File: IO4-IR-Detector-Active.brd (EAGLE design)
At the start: 50 x 50 mm, 32 parts, among them Q1 NPN-2222, Q2 NPN-2222, Q3 NPN-2222, Q4 NPN-2222

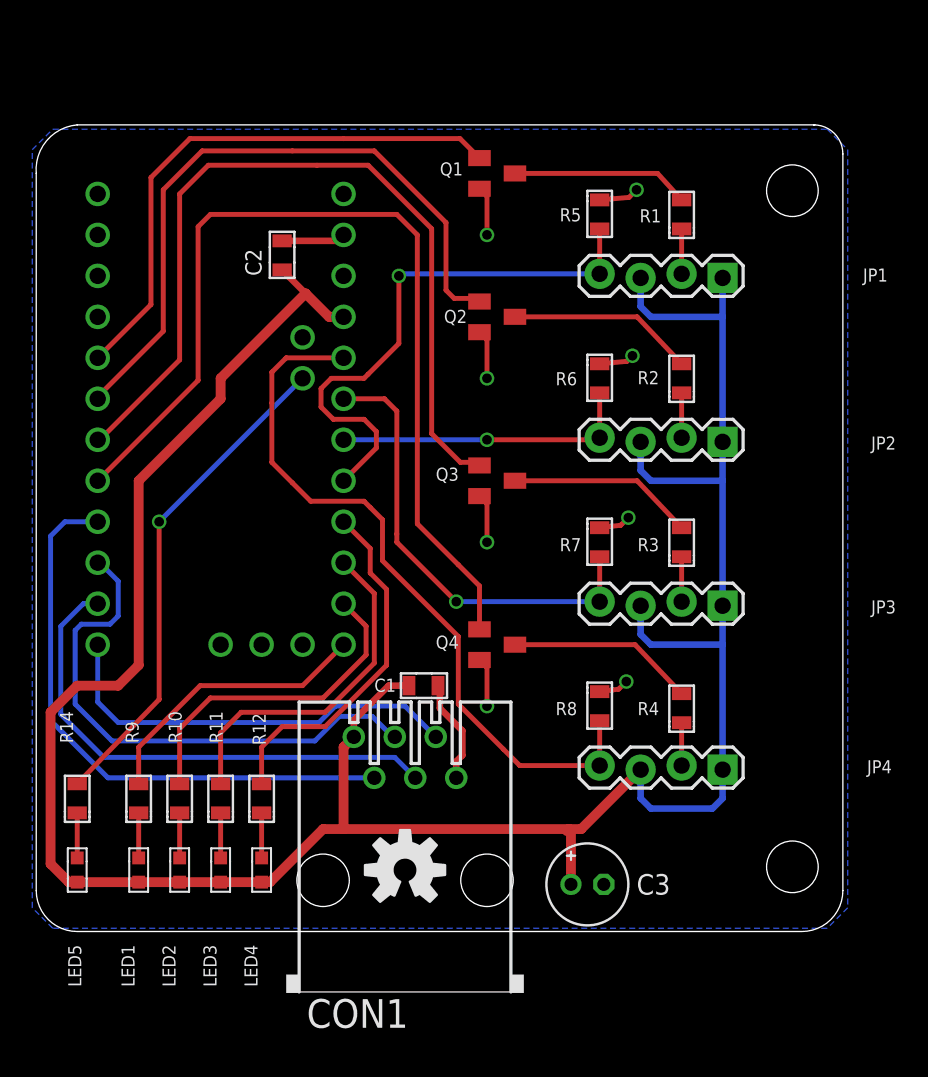
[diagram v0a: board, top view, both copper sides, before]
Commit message: panelized
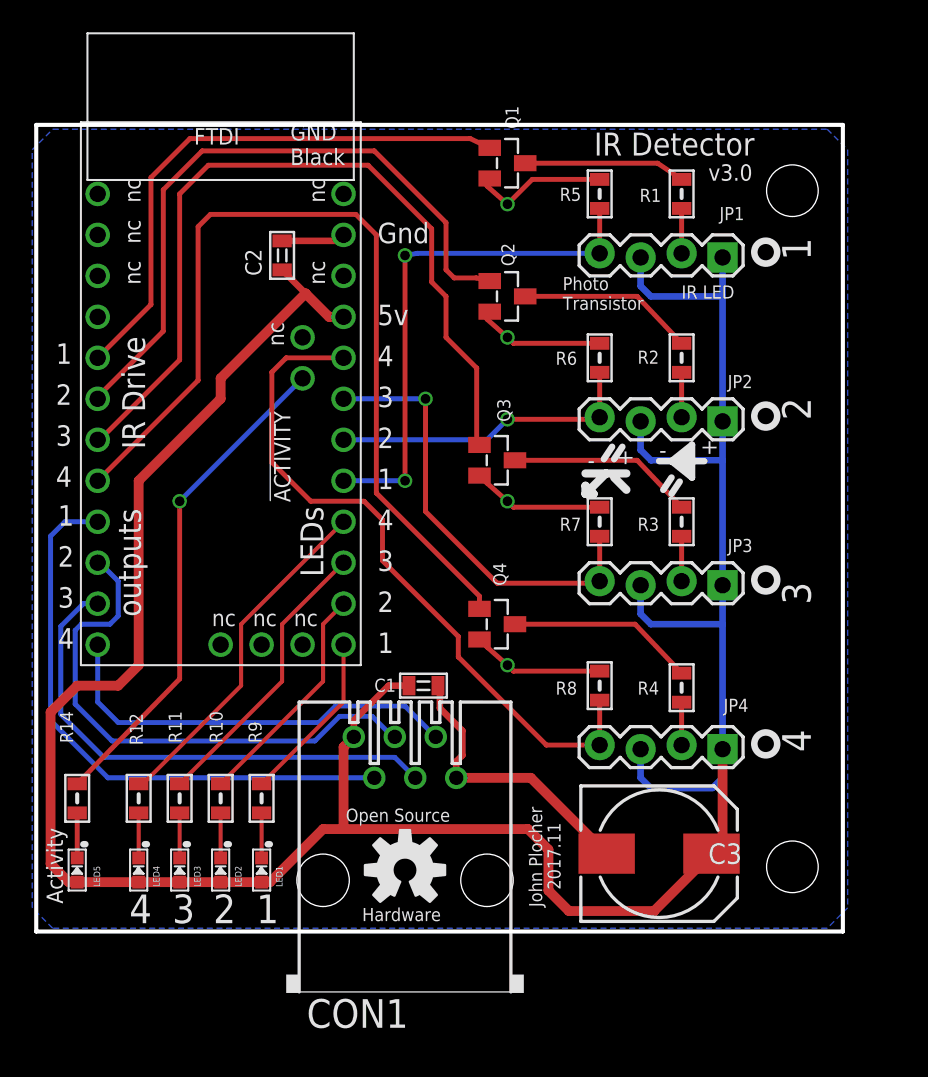
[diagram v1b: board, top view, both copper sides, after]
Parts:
- C3: device SPCoast:E2-5 -> SPCoast:0810-CAP
- moved LED1 7.62 mm to (14.0, 3.81), turned to 270 degrees
- moved LED4 7.62 mm to (6.35, 3.81), turned to 270 degrees
- moved R12 7.62 mm to (6.35, 8.26)
- moved R9 7.62 mm to (14.0, 8.26)
- moved C3 4.84 mm to (38.6, 4.83)
- moved LED2 2.54 mm to (11.4, 3.81), turned to 270 degrees
- moved LED3 2.54 mm to (8.89, 3.81), turned to 270 degrees
- moved R10 2.54 mm to (11.4, 8.26)
- moved R11 2.54 mm to (8.89, 8.26)
- moved Q2 1.42 mm to (29.2, 39.4), turned to 180 degrees
- moved R2 1.27 mm to (40.0, 35.6)
- moved R6 1.27 mm to (34.9, 35.6)
- moved JP2 1.27 mm to (42.5, 31.8)
- moved JP3 1.27 mm to (42.5, 21.6)
- moved JP4 1.27 mm to (42.5, 11.4)
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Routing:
- net GND: track 31.4 -> 54.8 mm, vias 8 -> 4
- net V+: track 164.3 -> 175.8 mm
- net L1: track 17.6 -> 10.7 mm
- net L2: track 20.6 -> 14.3 mm
- net L3: track 21.5 -> 17.9 mm
- net IR4: track 58.8 -> 56.0 mm
- net IRSIG4: track 45.2 -> 43.0 mm
- net IRSIG1: track 34.5 -> 32.6 mm, vias 1 -> 2
- net IR3: track 51.9 -> 50.0 mm
- net IRSIG3: track 28.6 -> 27.5 mm
- net IRDRIVE1: track 11.1 -> 10.0 mm
- net IR2: track 41.6 -> 40.9 mm
- net IRDRIVE2: track 11.6 -> 10.9 mm
- net IRSIG2: track 18.7 -> 19.2 mm
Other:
- outline, holes or cut-outs redrawn
- board text added: "C1"
- board text added: "C2"
- board text added: "C3"
- board text added: "CON1"
- board text added: "JP1"
- board text added: "JP2"
- board text added: "JP3"
- board text added: "JP4"
- board text added: "LED1"
- board text added: "LED2"
- board text added: "LED3"
- board text added: "LED4"
- board text added: "LED5"
- board text added: "Q1"
- board text added: "Q2"
- board text added: "Q3"
- board text added: "Q4"
- board text added: "R1"
- board text added: "R10"
- board text added: "R11"
- board text added: "R12"
- board text added: "R14"
- board text added: "R2"
- board text added: "R3"
- board text added: "R4"
- board text added: "R5"
- board text added: "R6"
- board text added: "R7"
- board text added: "R8"
- board text added: "R9"
